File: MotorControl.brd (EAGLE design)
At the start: 69 x 57 mm, 47 parts

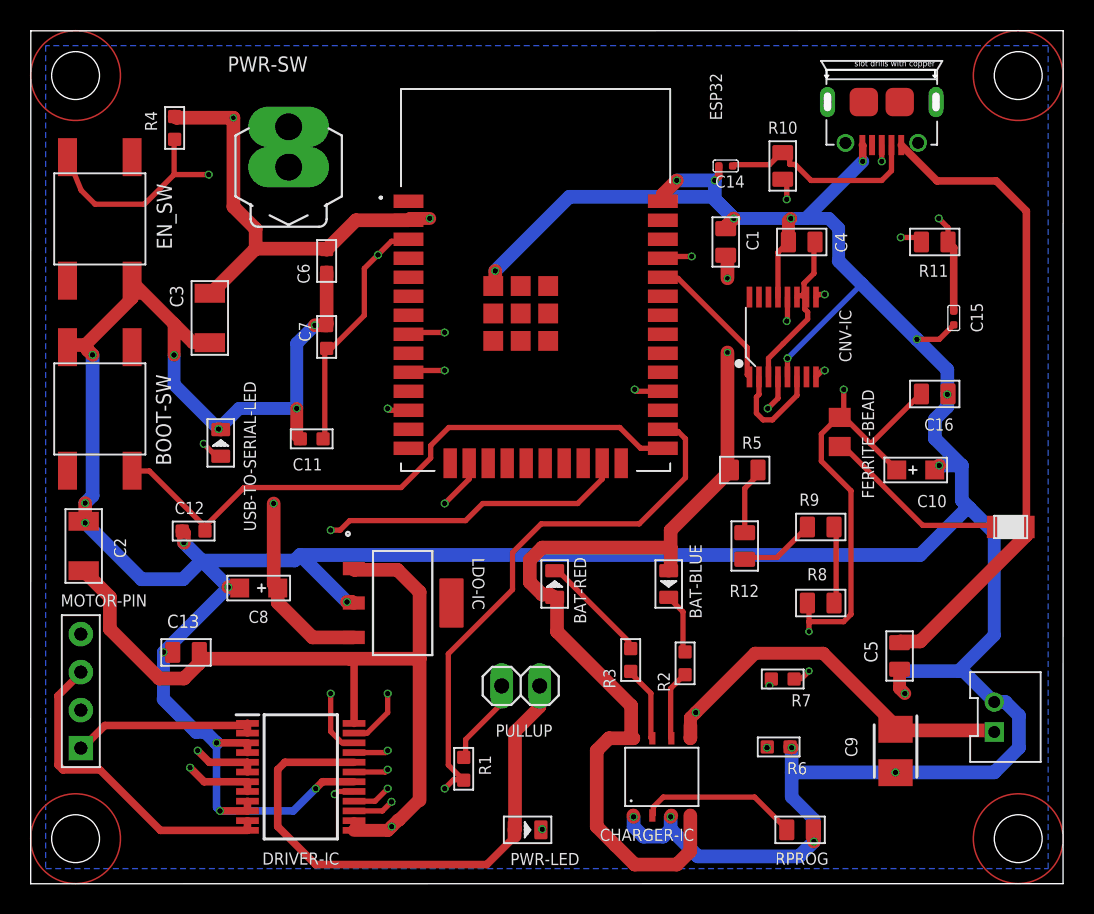
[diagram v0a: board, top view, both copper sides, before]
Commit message: [Modify] 部品置換前。在庫チェック中
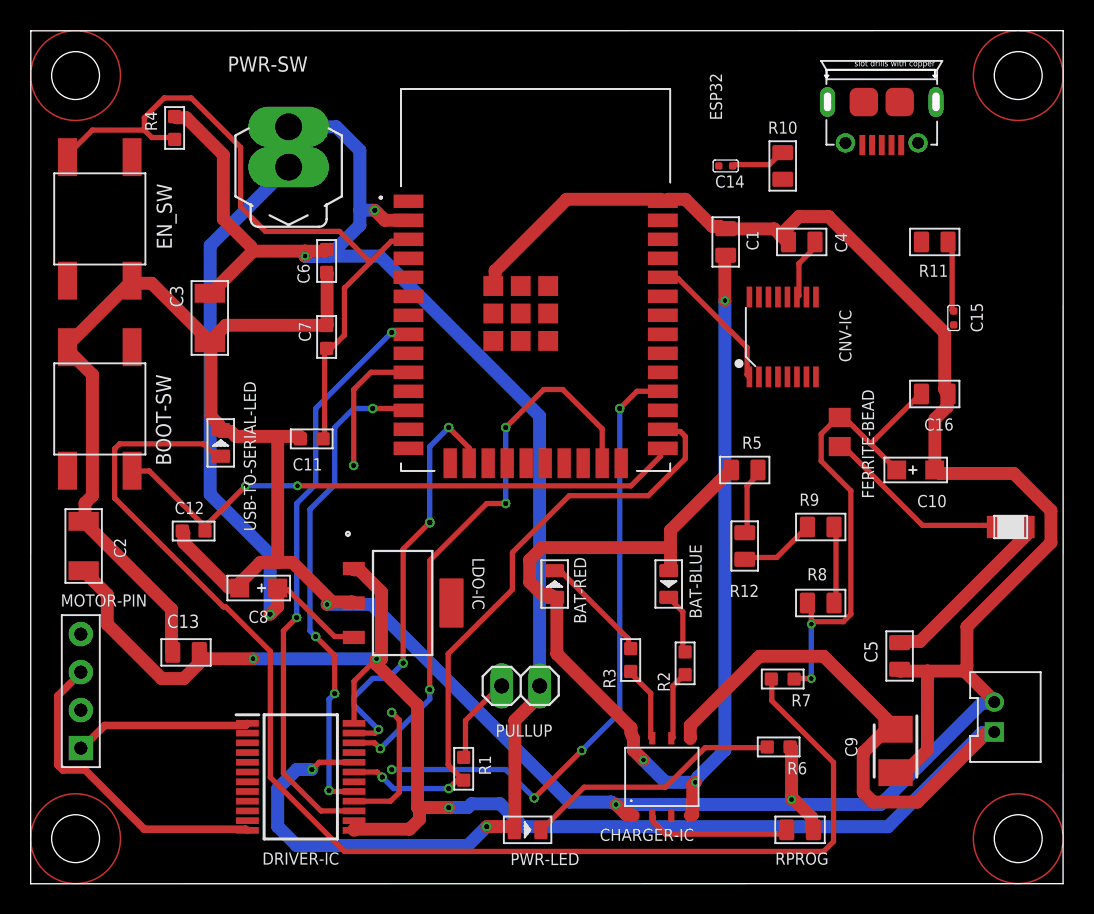
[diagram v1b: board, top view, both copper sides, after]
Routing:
- net GND: track 310.8 -> 231.5 mm, vias 30 -> 3
- net VBUS: track 43.4 -> 12.0 mm
- net B+: track 107.3 -> 130.9 mm, vias 2 -> 3
- net BO2: track 18.8 -> 0.00 mm, vias 1 -> 0
- net RXD: track 17.4 -> 0.00 mm, vias 2 -> 0
- net BIN2: track 35.2 -> 18.0 mm
- net N$8: track 13.3 -> 0.00 mm, vias 2 -> 0
- net AO2: track 13.2 -> 0.00 mm, vias 1 -> 0
- net VIN+: track 65.9 -> 77.6 mm, vias 2 -> 3
- net N$7: track 11.3 -> 0.00 mm, vias 2 -> 0
- net N$3: track 75.8 -> 86.6 mm, vias 2 -> 0
- net N$9: track 13.9 -> 3.72 mm
- net N$19: track 43.4 -> 33.9 mm, vias 4 -> 2
- net N$15: track 13.1 -> 4.80 mm, vias 2 -> 0
- net N$6: track 7.31 -> 0.00 mm
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- removed copper zone on layer 16, net GND
